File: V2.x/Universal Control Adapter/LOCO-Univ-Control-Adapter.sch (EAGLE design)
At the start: 28 parts, among them IC1 Atmega 328-P, IC2 MCP2515, IC4 LD117AS12TR, Q1 8MHz, Q2 16MHz

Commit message: Signed-off-by: Thomas Winkler <thomas.winkler@iggmp.net>
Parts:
- removed BUS: (no value), con-lstb:MA09-2
- removed C11, C5, C6, C8: 100n, rcl:C-EUC0402K
- removed C13: 16uF, rcl:CPOL-EUA/3216-18W
- removed C3, C4: 22p, rcl:C-EUC0402K
- removed CAN-1, CAN-2: 3-794618-4, SamacSys_Parts:3-794618-4
- removed DA1: TJA1050, TJA1050:TJA1050
- removed IC1: Atmega 328-P, atmel:MEGA8-AI
- removed IC2: MCP2515, mcp2514:MCP2515
- removed IC4: LD117AS12TR, v-reg:LD117AS12TR
- removed PWR: 22-23-2021, con-molex:22-23-2021
- removed Q1: 8MHz, crystal:CRYSTALHC49S
- removed Q2: 16MHz, crystal:CRYSTALHC49S
- removed R15: 10k, rcl:R-EU_MELF0102W
- removed SV1: (no value), con-lstb:MA05-1
- added AMP, BREAK, DIR, DRIVE, HORN, INSTR, LIGHT-1, MAINS, PWR/LIT-2, STATUS, V-BATT, V-MOT: (no value), jst-ph:JST-PH3
- added BUS1: (no value), con-lstb:MA09-1
- added BUS2A: (no value), con-lstb:MA05-1
- added BUS2B: (no value), con-lstb:MA04-1
- added IC5: LM340MP-05, linear:LM340MP-05
- added JP1: (no value), jumper:SJ2W
- added Q8: FDS5680, transistor-fet:FDS5680
- added R10, R11: 220R, rcl:R-EU_R0805
- added R12, R13: 10k, rcl:R-EU_R0603
- added R3, R4, R5: 10k, rcl:R-EU_R0805
- +5V: value (none) -> GRN
- C1: value 22p -> 100n
- C2: value 22p -> 16uF; device rcl:C-EUC0402K -> rcl:CPOL-EUA/3216-18W
- R1: device rcl:R-EU_MELF0102W -> rcl:R-EU_R0603
- R2: device rcl:R-EU_MELF0102W -> rcl:R-EU_R0805
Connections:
- removed net 12V-PWR: BUS.17, PWR-1.S
- removed net CAN-H: CAN-1.3, CAN-2.3, DA1.CANH
- removed net CAN-L: CAN-1.2, CAN-2.2, DA1.CANL
- removed net CAN-OCC1: C1.1, IC2.OSC1, Q1.1
- removed net CAN-OCC2: C2.1, IC2.OSC2, Q1.2
- removed net CS: IC1.PB2(SS/OC1B), IC2.!CS
- removed net DTR: C8.1, SV1.1
- removed net N$10: C3.1, IC1.PB6(XTAL1/TOSC1), Q2.1
- removed net N$11: C4.1, IC1.PB7(XTAL2/TOSC2), Q2.2
- removed net N$15: C8.2, IC1.PC6(/RESET), R2.1
- removed net N$6: IC2.!RST, R1.1
- removed net RX: IC1.PD1(TXD), SV1.3
- removed net RXCAN: DA1.RXD, IC2.RXCAN
- removed net SCK: IC1.PB5(SCK), IC2.SCK
- removed net SI: IC1.PB4(MISO), IC2.SO
- removed net SO: IC1.PB3(MOSI/OC2), IC2.SI
- removed net TX: IC1.PD0(RXD), SV1.2
- removed net TXCAN: DA1.TXD, IC2.TXCAN
- new net GREEN: R11.2, STATUS.3
- new net INSTR-LIGHT: INSTR.2, Q8.D
- new net N$2: BUS2A.1
- new net N$8: Q8.G, R12.1, R13.2
- new net RED: R10.2, STATUS.1
- new net SUPL: INSTR.1, JP1.2
- net +12V: now also C1.2, C2.+, IC5.VI, JP1.1; no longer C11.2, C13.+, CAN-1.4, CAN-2.4, IC4.IN
- net A0: now also BUS2B.2, DRIVE.2; no longer BUS.13, IC1.PC0(ADC0)
- net A1: now also BREAK.2, BUS2B.1; no longer BUS.11, IC1.PC1(ADC1)
- net A2: now also BUS2A.5, PWR/LIT-2.2; no longer BUS.9, IC1.PC2(ADC2)
- net A3: now also BUS2A.4, DIR.2, R2.1, R3.1; no longer BUS.7, IC1.PC3(ADC3)
- net A4: now also BUS2A.3, MAINS.2, R4.1, R5.1; no longer BUS.5, IC1.PC4(ADC4/SDA)
- net A5: now also BUS2A.2, LIGHT-1.2; no longer BUS.3, IC1.PC5(ADC5/SCL)
- net D2: now also BUS1.2, R10.1; no longer BUS.2, IC1.PD2(INT0)
- net D3: now also BUS1.3, R11.1; no longer BUS.4, IC1.PD3(INT1)
- net D4: now also BUS1.4, R12.2; no longer BUS.6, IC1.PD4(XCK/T0)
- net D5: now also BUS1.5, HORN.1; no longer BUS.8, IC1.PD5(T1)
- net D6: now also BUS1.6, V-BATT.1; no longer BUS.10, IC1.PD6(AIN0)
- net D7: now also BUS1.7, V-MOT.1; no longer BUS.12, IC1.PD7(AIN1)
- net D8: now also AMP.1, BUS1.8; no longer BUS.14, IC1.PB0(ICP)
- net D9: now also BUS2B.3, HORN.2; no longer BUS.15, IC1.PB1(OC1A)
- net GND: now also AMP.3, BREAK.1, BUS1.9, BUS2B.4, C1.1, C2.-, DIR.1, DRIVE.1, HORN.3, IC5.GND, INSTR.3, LIGHT-1.1, MAINS.1, PWR/LIT-2.1, Q8.S, R1.1, R13.1, R3.2, R5.2, STATUS.2, V-BATT.3, V-MOT.3; no longer BUS.16, BUS.18, C1.2, C11.1, C13.-, C2.2, C3.2, C4.2, C5.1, C6.2, CAN-1.1, CAN-2.1, DA1.RS, DA1.VSS, IC1.GND@1, IC2.VSS, IC4.ADJ, PWR-2.S, R15.1, SV1.5
- net N$12: now also R1.2; no longer R15.2
- net VCC: now also AMP.2, BREAK.3, DIR.3, DRIVE.3, IC5.VO, JP1.3, LIGHT-1.3, MAINS.3, PWR/LIT-2.3, R4.2, V-BATT.2, V-MOT.2; no longer BUS.1, C5.2, C6.1, DA1.VDD, IC1.AVCC, IC1.VCC@1, IC2.VDD, IC4.OUT, R1.2, SV1.4
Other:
- note added: "LOCO-Control-Adapter V2.1"
- note removed: "CAN-Interface"
- note removed: "Controler"
- note removed: "IFTDI-Interface"

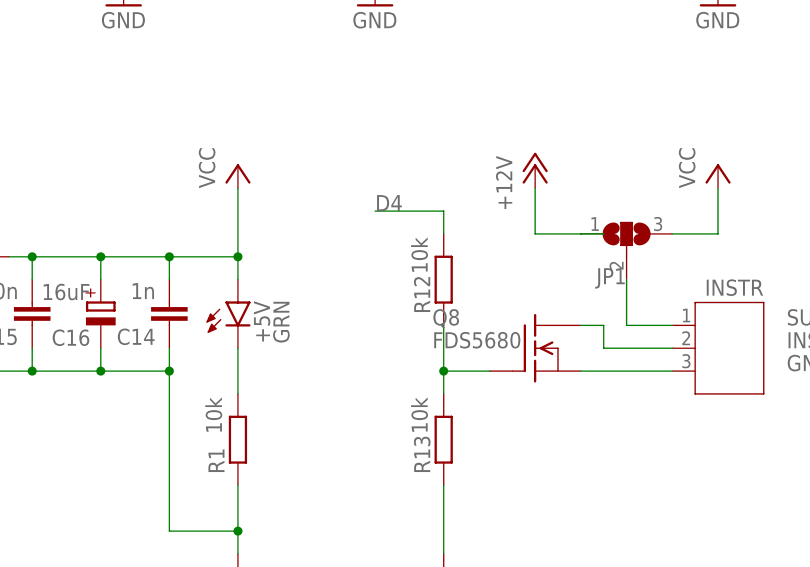
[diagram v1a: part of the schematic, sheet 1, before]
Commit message: initial
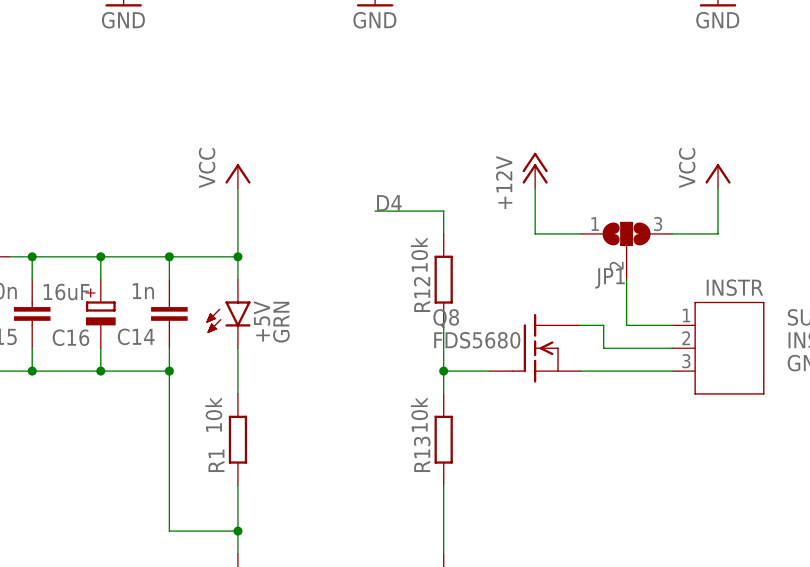
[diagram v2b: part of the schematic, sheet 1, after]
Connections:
- removed net N$2: BUS2A.1
- net +12V: now also BUS2A.1
